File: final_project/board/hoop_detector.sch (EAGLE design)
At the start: 59 parts

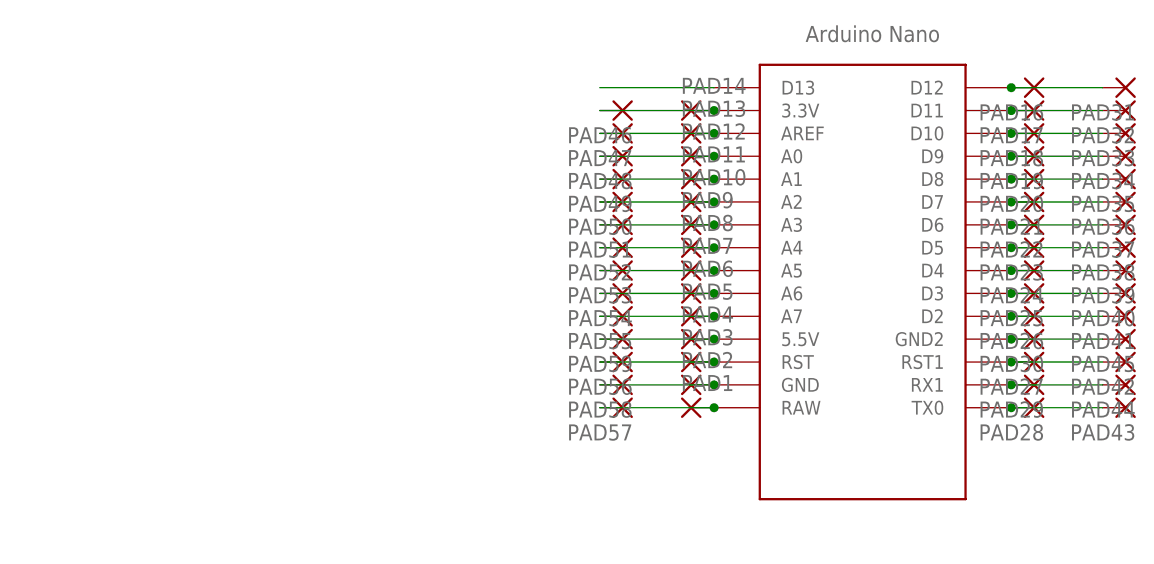
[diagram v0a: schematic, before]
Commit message: board
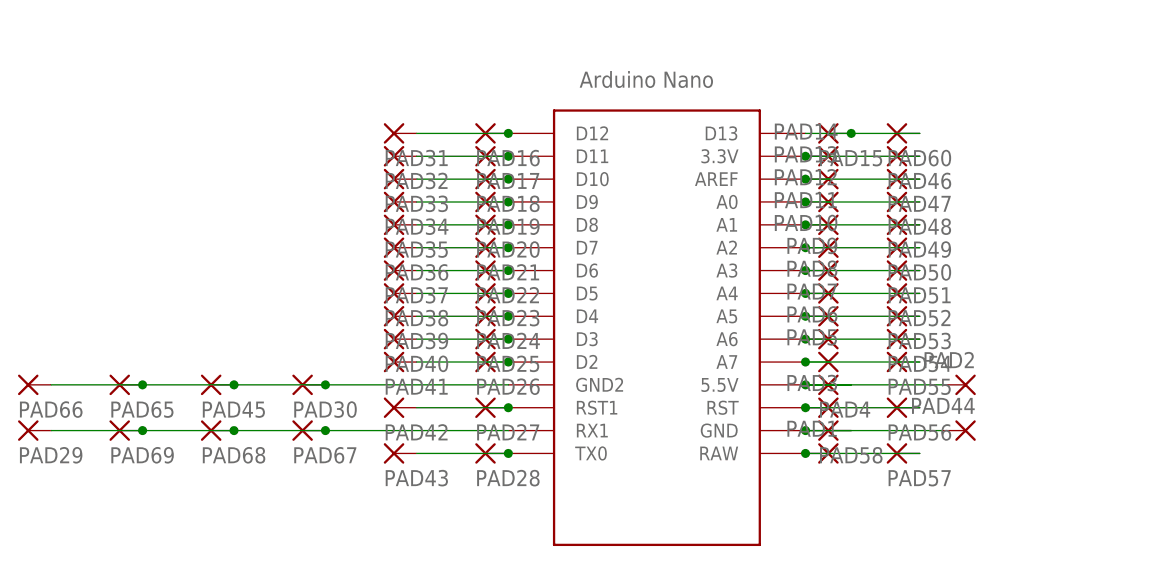
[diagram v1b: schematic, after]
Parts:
- removed PAD59: (no value), wirepad:1,6/0,9
- added PAD15, PAD60, PAD65, PAD66, PAD67, PAD68, PAD69: (no value), wirepad:1,6/0,9
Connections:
- net N$12: now also PAD67.P, PAD68.P, PAD69.P; no longer PAD44.P
- net N$13: now also PAD65.P, PAD66.P
- net N$16: now also PAD15.P, PAD60.P
- net N$27: now also PAD2.P; no longer PAD59.P
- net N$29: now also PAD44.P; no longer PAD2.P
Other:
- moved on the sheet: PAD1, PAD10, PAD11, PAD12, PAD13, PAD14, PAD16, PAD17, PAD18, PAD19, PAD2, PAD20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
